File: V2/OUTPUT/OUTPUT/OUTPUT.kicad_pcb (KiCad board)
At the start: 2 copper layers, 100 x 30 mm, 32 parts, among them J1 Conn_01x03, J2 Conn_01x03, J3 Conn_01x03, J4 Conn_01x03, J5 Conn_01x03, J6 Conn_01x03, J7 Conn_01x03, J8 Conn_01x03, Q1 QM6006D, Q2 QM6006D, Q3 QM6006D, Q4 QM6006D, Q5 QM6006D, Q6 QM6006D, Q7 QM6006D, Q8 QM6006D

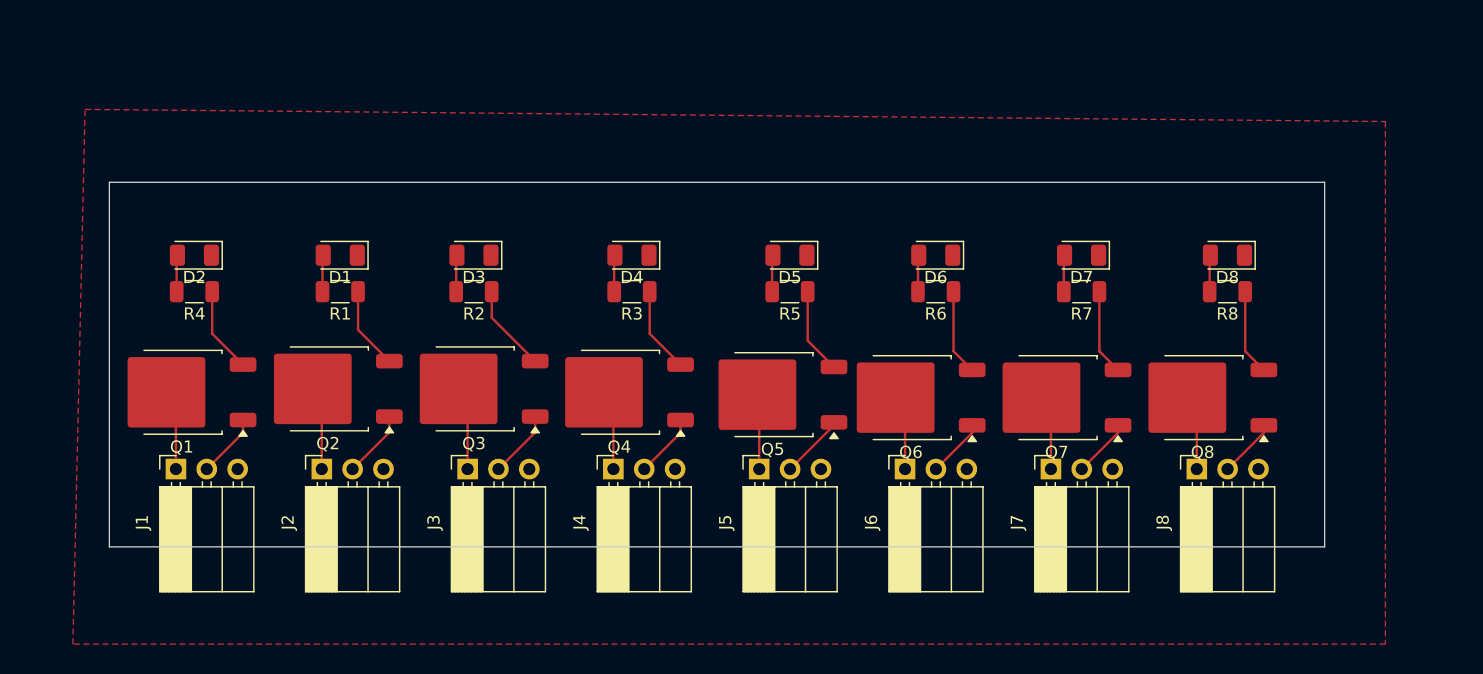
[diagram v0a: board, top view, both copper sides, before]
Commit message: Auto-update: 29.03.2026  0:17:51,75
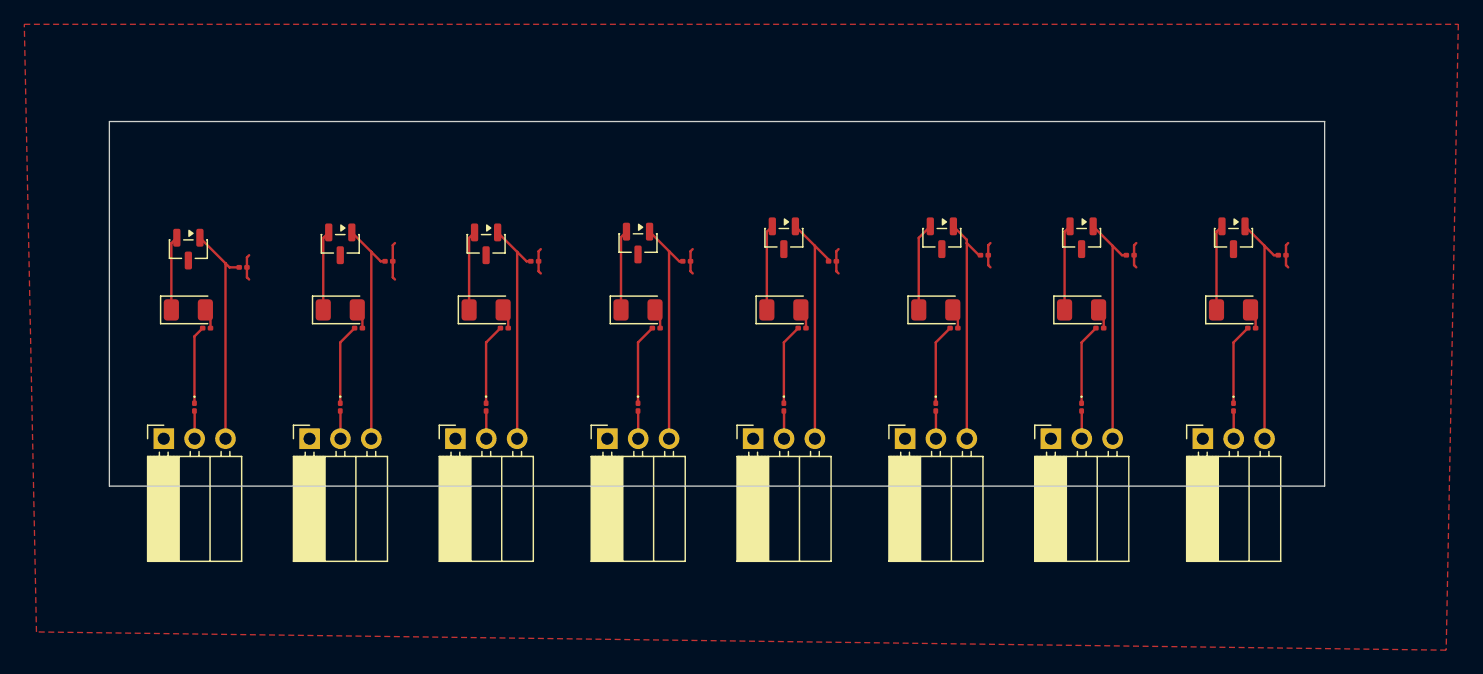
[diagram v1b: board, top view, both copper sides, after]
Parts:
- added D10: D_Zener, Diode_SMD:D_0201_0603Metric, F.Cu at (55.5, 23.5)
- added D11: LED, LED_SMD:LED_1206_3216Metric, F.Cu at (68.0, 15.5)
- added D12: D_Zener, Diode_SMD:D_0201_0603Metric, F.Cu at (68.0, 23.5)
- added D13: LED, LED_SMD:LED_1206_3216Metric, F.Cu at (80.0, 15.5)
- added D14: D_Zener, Diode_SMD:D_0201_0603Metric, F.Cu at (80.0, 23.5)
- added D15: LED, LED_SMD:LED_1206_3216Metric, F.Cu at (92.5, 15.5)
- added D16: D_Zener, Diode_SMD:D_0201_0603Metric, F.Cu at (92.5, 23.5)
- added D9: LED, LED_SMD:LED_1206_3216Metric, F.Cu at (55.5, 15.5)
- added R10: 10k, Resistor_SMD:R_0201_0603Metric, F.Cu at (59.5, 11.5)
- added R11: R, Resistor_SMD:R_0201_0603Metric, F.Cu at (69.5, 17.0)
- added R12: 10k, Resistor_SMD:R_0201_0603Metric, F.Cu at (72.0, 11.0)
- added R13: R, Resistor_SMD:R_0201_0603Metric, F.Cu at (81.5, 17.0)
- added R14: 10k, Resistor_SMD:R_0201_0603Metric, F.Cu at (84.0, 11.0)
- added R15: R, Resistor_SMD:R_0201_0603Metric, F.Cu at (94.0, 17.0)
- added R16: 10k, Resistor_SMD:R_0201_0603Metric, F.Cu at (96.5, 11.0)
- added R9: R, Resistor_SMD:R_0201_0603Metric, F.Cu at (57.0, 17.0)
- D3, D4, D6, D8: value LED -> D_Zener; footprint LED_SMD:LED_1206_3216Metric -> Diode_SMD:D_0201_0603Metric
- Q1, Q2, Q3, Q4, Q5, Q6, Q7, Q8: footprint Package_TO_SOT_SMD:TO-252-2 -> Package_TO_SOT_SMD:SOT-23
- R1, R3, R6, R8: value R -> 10k; footprint Resistor_SMD:R_1206_3216Metric -> Resistor_SMD:R_0201_0603Metric
- R2, R4, R5, R7: footprint Resistor_SMD:R_1206_3216Metric -> Resistor_SMD:R_0201_0603Metric
- moved D8 50.1 mm to (43.5, 23.5), turned to -90 degrees
- moved R8 44.6 mm to (47.5, 11.5), turned to 0 degrees
- moved D6 39.1 mm to (31.0, 23.5), turned to -90 degrees
- moved D7 36.8 mm to (43.5, 15.5), turned to 0 degrees
- moved R7 35.1 mm to (45.0, 17.0), turned to 0 degrees
- moved R6 33.1 mm to (35.0, 11.5), turned to 0 degrees
- moved D4 27.1 mm to (19.0, 23.5), turned to -90 degrees
- moved D3 26.2 mm to (7.00, 23.5), turned to -90 degrees
- moved D5 25.4 mm to (31.0, 15.5), turned to 0 degrees
- moved R5 23.7 mm to (32.5, 17.0), turned to 0 degrees
- moved R3 20.2 mm to (23.0, 11.5), turned to 0 degrees
- moved Q6 13.4 mm to (68.5, 9.56), turned to -90 degrees
- moved Q8 13.4 mm to (92.5, 9.56), turned to -90 degrees
- moved Q7 13.3 mm to (80.0, 9.56), turned to -90 degrees
- moved Q5 12.9 mm to (55.5, 9.56), turned to -90 degrees
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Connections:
- D1 pad 1: GND -> Net-(D1-K)
- D2 pad 1: GND -> Net-(D2-K)
- D3 pad 1: GND -> Net-(D3-K)
- D3 pad 2: Net-(D3-A) -> +5V
- D4 pad 1: GND -> Net-(D4-K)
- D4 pad 2: Net-(D4-A) -> +5V
- D5 pad 1: GND -> Net-(D5-K)
- D6 pad 1: GND -> Net-(D6-K)
- D6 pad 2: Net-(D6-A) -> +5V
- D7 pad 1: GND -> Net-(D7-K)
- D8 pad 1: GND -> Net-(D8-K)
- D8 pad 2: Net-(D8-A) -> +5V
- J1 pad 1: +5V -> GND
- J1 pad 2: Net-(J1-Pin_2) -> +5V
- J1 pad 3: GND -> Net-(J1-Pin_3)
- J2 pad 1: +5V -> GND
- J2 pad 2: Net-(J2-Pin_2) -> +5V
- J2 pad 3: GND -> Net-(J2-Pin_3)
- J3 pad 1: +5V -> GND
- J3 pad 2: Net-(J3-Pin_2) -> +5V
- J3 pad 3: GND -> Net-(J3-Pin_3)
- J4 pad 1: +5V -> GND
- J4 pad 2: Net-(J4-Pin_2) -> +5V
- J4 pad 3: GND -> Net-(J4-Pin_3)
- J5 pad 1: +5V -> GND
- J5 pad 2: Net-(J5-Pin_2) -> +5V
- J5 pad 3: GND -> Net-(J5-Pin_3)
- J6 pad 1: +5V -> GND
- J6 pad 2: Net-(J6-Pin_2) -> +5V
- J6 pad 3: GND -> Net-(J6-Pin_3)
- J7 pad 1: +5V -> GND
- J7 pad 2: Net-(J7-Pin_2) -> +5V
- J7 pad 3: GND -> Net-(J7-Pin_3)
- J8 pad 1: +5V -> GND
- J8 pad 2: Net-(J8-Pin_2) -> +5V
- J8 pad 3: GND -> Net-(J8-Pin_3)
- Q1 pad 1: Net-(J1-Pin_2) -> Net-(J1-Pin_3)
- Q1 pad 2: +5V -> Net-(D2-K)
- Q1 pad 3: Net-(Q1-S) -> GND
- Q2 pad 1: Net-(J2-Pin_2) -> Net-(J2-Pin_3)
- Q2 pad 2: +5V -> Net-(D1-K)
- Q2 pad 3: Net-(Q2-S) -> GND
- Q3 pad 1: Net-(J3-Pin_2) -> Net-(J3-Pin_3)
- Q3 pad 2: +5V -> Net-(D5-K)
- Q3 pad 3: Net-(Q3-S) -> GND
- Q4 pad 1: Net-(J4-Pin_2) -> Net-(J4-Pin_3)
- Q4 pad 2: +5V -> Net-(D7-K)
- Q4 pad 3: Net-(Q4-S) -> GND
- Q5 pad 1: Net-(J5-Pin_2) -> Net-(J5-Pin_3)
- Q5 pad 2: +5V -> Net-(D9-K)
- Q5 pad 3: Net-(Q5-S) -> GND
- Q6 pad 1: Net-(J6-Pin_2) -> Net-(J6-Pin_3)
- Q6 pad 2: +5V -> Net-(D11-K)
- Q6 pad 3: Net-(Q6-S) -> GND
- Q7 pad 1: Net-(J7-Pin_2) -> Net-(J7-Pin_3)
- Q7 pad 2: +5V -> Net-(D13-K)
- Q7 pad 3: Net-(Q7-S) -> GND
- Q8 pad 1: Net-(J8-Pin_2) -> Net-(J8-Pin_3)
- Q8 pad 2: +5V -> Net-(D15-K)
- Q8 pad 3: Net-(Q8-S) -> GND
- R1 pad 1: Net-(Q2-S) -> Net-(J1-Pin_3)
- R1 pad 2: Net-(D1-A) -> GND
- R2 pad 1: Net-(Q3-S) -> Net-(D4-K)
- R2 pad 2: Net-(D3-A) -> Net-(D1-A)
- R3 pad 1: Net-(Q4-S) -> Net-(J2-Pin_3)
- R3 pad 2: Net-(D4-A) -> GND
- R4 pad 1: Net-(Q1-S) -> Net-(D3-K)
- R5 pad 1: Net-(Q5-S) -> Net-(D6-K)
- R6 pad 1: Net-(Q6-S) -> Net-(J3-Pin_3)
- R6 pad 2: Net-(D6-A) -> GND
- R7 pad 1: Net-(Q7-S) -> Net-(D8-K)
- R8 pad 1: Net-(Q8-S) -> Net-(J4-Pin_3)
- R8 pad 2: Net-(D8-A) -> GND
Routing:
- net +5V: track 51.9 -> 18.3 mm
- net Net-(J5-Pin_3): track 0.00 -> 19.9 mm
- net Net-(J8-Pin_3): track 0.00 -> 19.6 mm
- net Net-(J7-Pin_3): track 0.00 -> 19.6 mm
- net Net-(J6-Pin_3): track 0.00 -> 19.5 mm
- net Net-(J4-Pin_3): track 0.00 -> 19.2 mm
- net Net-(J2-Pin_3): track 0.00 -> 19.1 mm
- net Net-(J3-Pin_3): track 0.00 -> 19.1 mm
- net Net-(J1-Pin_3): track 0.00 -> 18.7 mm
- net GND: track 0.00 -> 18.2 mm
- net Net-(D11-K): track 0.00 -> 7.27 mm
- net Net-(Q3-S): track 7.20 -> 0.00 mm
- net Net-(Q5-S): track 7.09 -> 0.00 mm
- net Net-(Q8-S): track 7.08 -> 0.00 mm
- net Net-(Q7-S): track 7.08 -> 0.00 mm
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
